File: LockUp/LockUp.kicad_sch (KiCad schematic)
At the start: 41 parts, among them J2 Motor, J4 Key_Sw, J5 DND_sw, J7 Servo, Q1 AO3401A, Q3 AO3400A, U1 ESP32-C6-WROOM-1, U2 L9110S, U3 MFRC522{slash}RC522, U4 L9110S

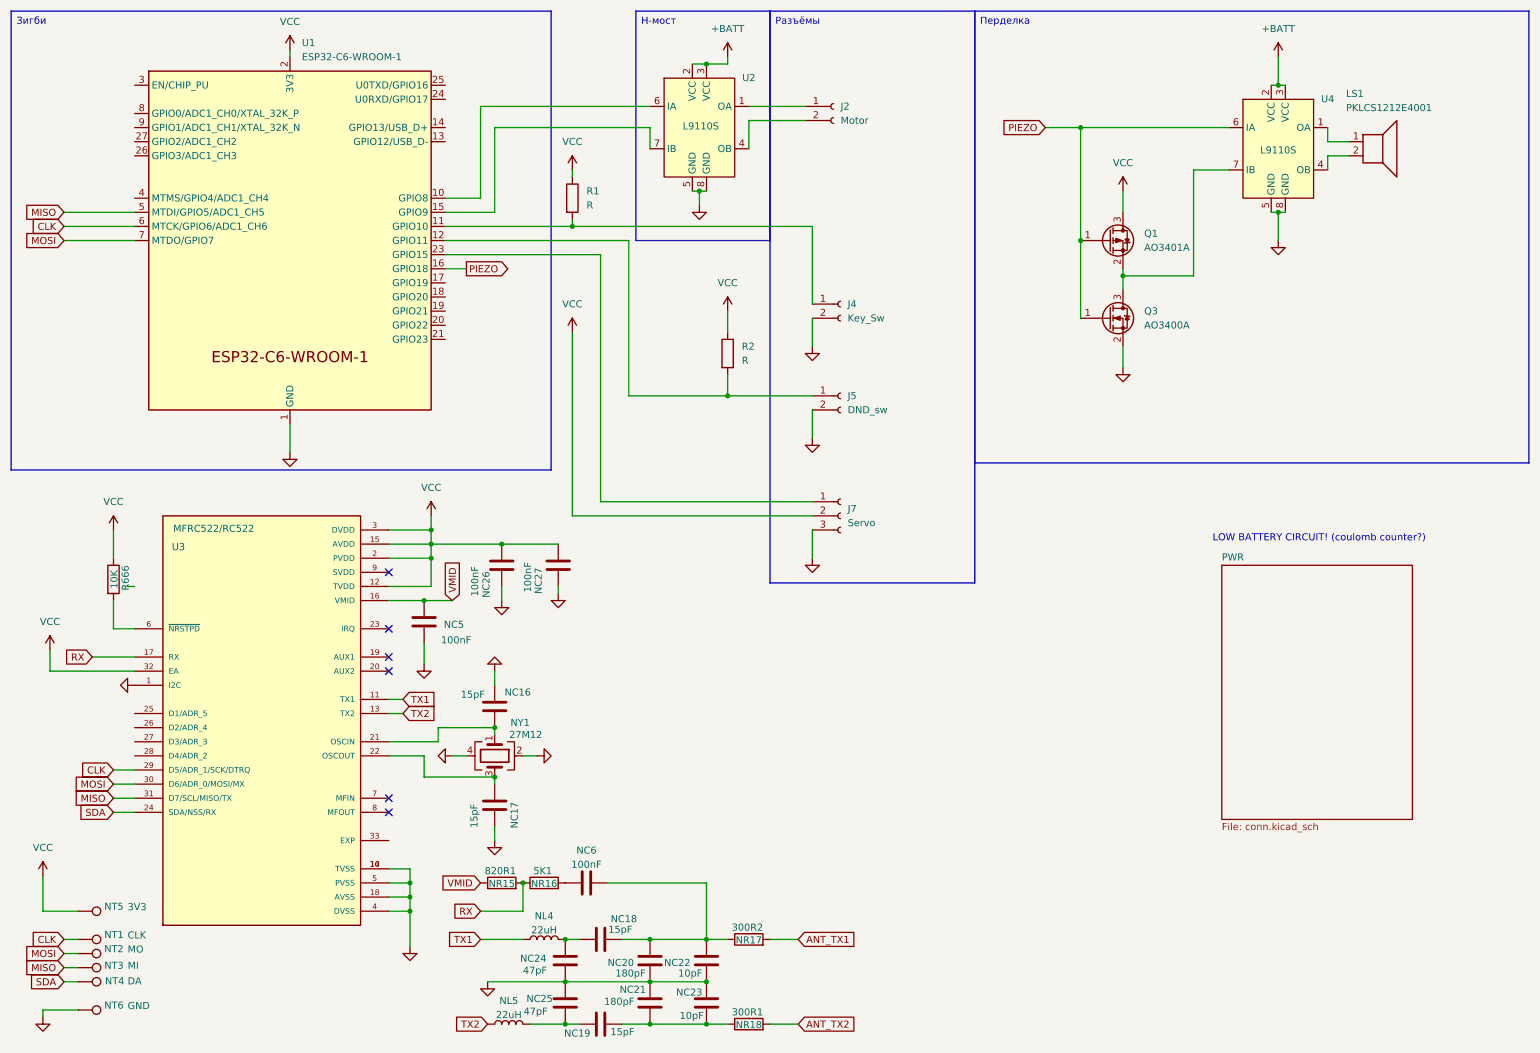
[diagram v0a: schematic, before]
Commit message: bat mon done
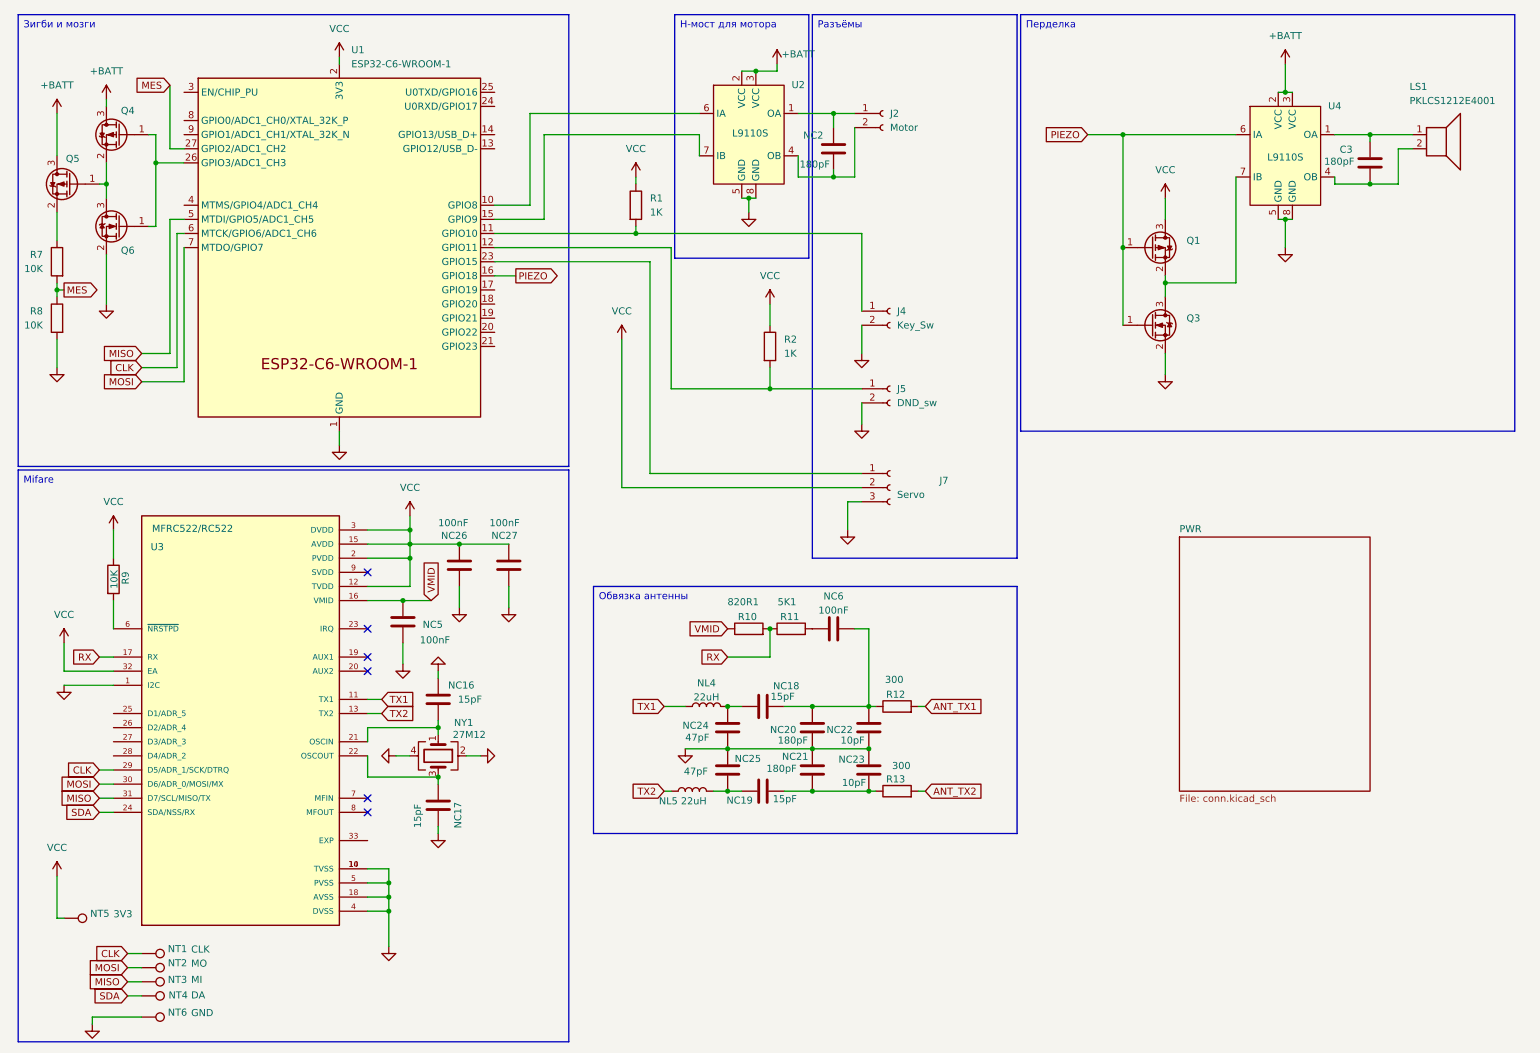
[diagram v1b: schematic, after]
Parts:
- removed Q1: AO3401A, Package_TO_SOT_SMD:SOT-23, symbol Transistor_FET:AO3401A
- added C3, NC2: 180pF, Capacitor_SMD:C_0805_2012Metric_Pad1.18x1.45mm_HandSolder, symbol Device:C
- added Q1, Q4, Q5: Si2323, Package_TO_SOT_SMD:SOT-23, symbol OrnexParts:Si2323
- added Q6: AO3400A, Package_TO_SOT_SMD:SOT-23, symbol Transistor_FET:AO3400A
- added R7, R8: 10K, Resistor_SMD:R_0805_2012Metric_Pad1.20x1.40mm_HandSolder, symbol Device:R
- R1, R2: value R -> 1K; footprint (none) -> Resistor_SMD:R_0805_2012Metric_Pad1.20x1.40mm_HandSolder
- R10: renamed from 820R1; value NR15 -> 820R1
- R11: renamed from 5K1; value NR16 -> 5K1
- R12: renamed from 300R2; value NR17 -> 300
- R13: renamed from 300R1; value NR18 -> 300
- renumbered R666 to R9
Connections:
- net +BATT: now also Q4.3 (D), Q5.3 (D)
- net GND: now also Q6.2 (S), R8.2
- net PIEZO: now also Q1.1 (G)
- net VCC: now also Q1.3 (D)
- net at U1.26 (GPIO3/ADC1_CH3): now also Q4.1 (G), Q6.1 (G)
- net MES: now reaches U1.27 (GPIO2/ADC1_CH2)
- net MES: now also R7.2, R8.1
- net at Q3.3 (D), U4.7 (IB): now also Q1.2 (S)
- net at J2.1 (Pin_1), U2.1 (OA): now also NC2.1
- net at J2.2 (Pin_2), U2.4 (OB): now also NC2.2
- net at LS1.1, U4.1 (OA): now also C3.1
- net at LS1.2, U4.4 (OB): now also C3.2
- new net: Q4.2 (S), Q5.1 (G), Q6.3 (D)
- new net: Q5.2 (S), R7.1
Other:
- note removed: "LOW BATTERY CIRCUIT! (coulomb counter?)"
- company: (none) -> Ornex
- title: (none) -> Ornex Z-Lock
- moved on the sheet: J2, J4, J5, J7, LS1, NC16, NC17, NC18, NC19, NC20, NC21, NC22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
